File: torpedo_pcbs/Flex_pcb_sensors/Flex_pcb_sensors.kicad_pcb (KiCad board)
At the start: 2 copper layers, 38.2 x 23.8 mm, 9 parts, among them IC1 VL53L1CXV0FY_1, J1 Conn_01x04, J2 Conn_01x04, U1 MS583702BA01-50

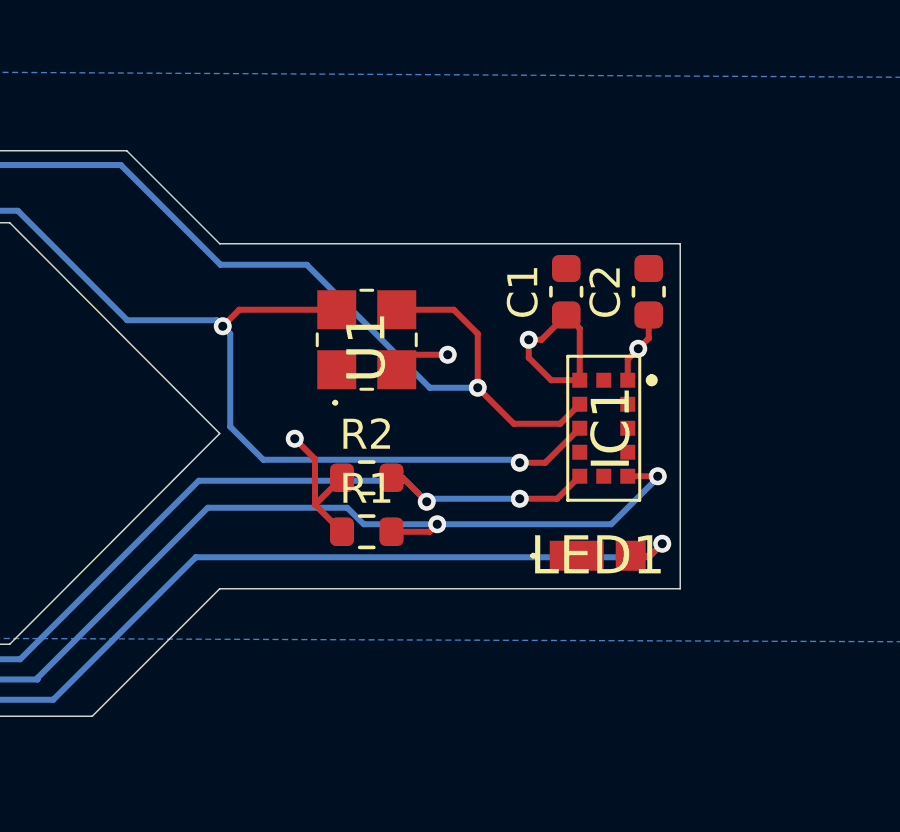
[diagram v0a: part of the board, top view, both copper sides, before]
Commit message: flex_pcb_updates
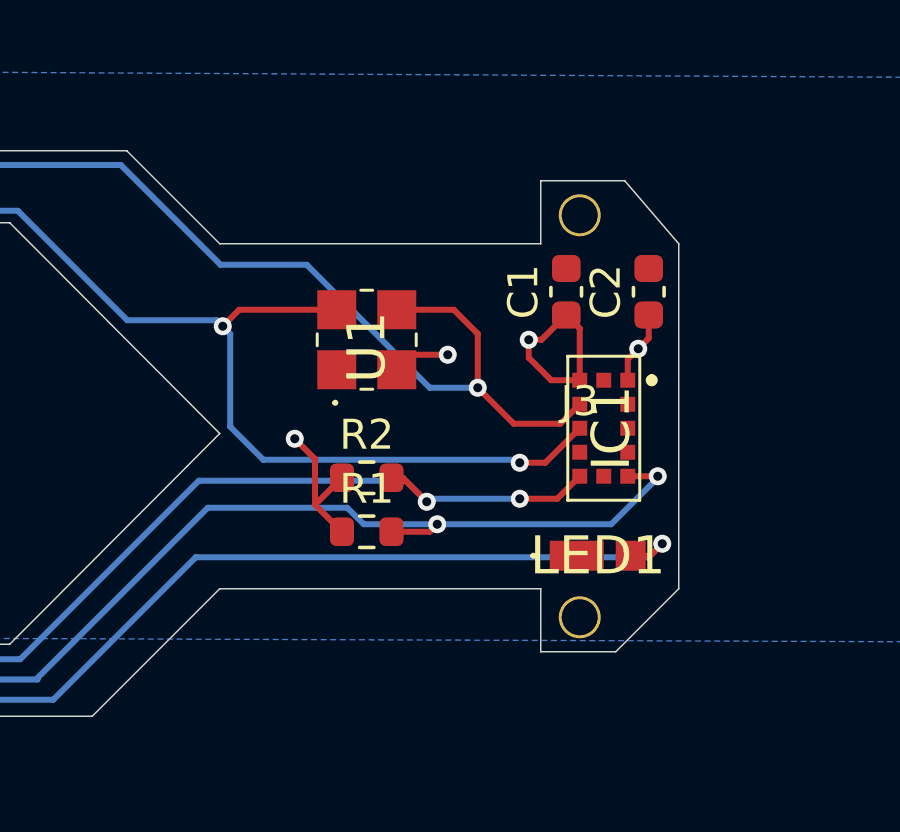
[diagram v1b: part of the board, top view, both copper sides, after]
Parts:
- added J3: mounting, MountingEquipment:small mounting holes, F.Cu at (171.8, 79.5)
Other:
- board size 38.2 x 23.8 mm -> 38.1 x 23.8 mm
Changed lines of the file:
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@@
 	(net 8 "unconnected-(J1-Pin_4-Pad4)")
 	(net 9 "Net-(J1-Pin_3)")
+	(footprint "MountingEquipment:small mounting holes"
+		(layer "F.Cu")
+		(at 171.8 79.45)
+		(property "Reference" "J3"
+			(at 0 -0.5 0)
+			(unlocked yes)
+			(layer "F.SilkS")
+			(effects
+				(font
+					(size 1 1)
+					(thickness 0.1)
+				)
+			)
+		)
+		(property "Value" "mounting"
+			(at 0 1 0)
+			(unlocked yes)
+			(layer "F.Fab")
+			(effects
+				(font
+					(size 1 1)
+					(thickness 0.15)
+				)
+			)
+		)
+		(property "Footprint" "MountingEquipment:small mounting holes"
+			(at 0 0 0)
+			(unlocked yes)
+			(layer "F.Fab")
+			(hide yes)
+			(effects
+				(font
+					(size 1 1)
+					(thickness 0.15)
+				)
+			)
+		)
+		(property "Datasheet" ""
+			(at 0 0 0)
+			(unlocked yes)
+			(layer "F.Fab")
+			(hide yes)
+			(effects
+				(font
+					(size 1 1)
+					(thickness 0.15)
+				)
+			)
+		)
+		(property "Description" "Generic connector, single row, 01x02, script generated (kicad-library-utils/schlib/autogen/connector/)"
+			(at 0 0 0)
+			(unlocked yes)
+			(layer "F.Fab")
+			(hide yes)
+			(effects
+				(font
+					(size 1 1)
+					(thickness 0.15)
+				)
+			)
+		)
+		(property ki_fp_filters "Connector*:*_1x??_*")
+		(sheetname "Root")
+		(sheetfile "Flex_pcb_sensors.kicad_sch")
+		(attr through_hole)
+		(fp_text user "${REFERENCE}"
+			(at 0 2.5 0)
+			(unlocked yes)
+			(layer "F.Fab")
+			(effects
+				(font
+					(size 1 1)
+					(thickness 0.15)
+				)
+			)
+		)
+		(pad "1" thru_hole circle
+			(at 0 -6.7)
+			(size 1.4 1.4)
+			(drill 1.2)
+			(layers "*.Cu" "*.Mask")
+			(remove_unused_layers no)
+			(net 4 "GND")
+			(pinfunction "Pin_1")
+			(pintype "passive")
+			(thermal_bridge_angle 90)
+		)
+		(pad "2" thru_hole circle
+			(at 0 6.7)
+			(size 1.4 1.4)
+			(drill 1.2)
+			(layers "*.Cu" "*.Mask")
+			(remove_unused_layers no)
+			(net 4 "GND")
+			(pinfunction "Pin_2")
+			(pintype "passive")
+			(thermal_bridge_angle 90)
+		)
+	)
 	(footprint "SamacSys_Parts:MS583702BA0150"
 		(layer "F.Cu")
@@
 		(tags "LED")
 		(property "Reference" "LED1"
-			(at 0 0 360)
+			(at 0 0 0)
 			(layer "F.SilkS")
 			(effects
@@
 		)
 		(property "Value" "158301260A"
-			(at 0 0 360)
+			(at 0 0 0)
 			(layer "F.SilkS")
 			(hide yes)
@@
 		)
 		(fp_line
-			(start -2.600001 1.7)
+			(start -2.6 -1.7)
+			(end 2.6 -1.7)
+			(stroke
+				(width 0.1)
+				(type solid)
+			)
+			(layer "F.CrtYd")
+		)
+		(fp_line
+			(start -2.6 1.7)
 			(end -2.6 -1.7)
 			(stroke
@@
 		)
 		(fp_line
-			(start -2.6 -1.7)
-			(end 2.600001 -1.7)
+			(start 2.6 -1.7)
+			(end 2.6 1.7)
 			(stroke
 				(width 0.1)
@@
 		(fp_line
 			(start 2.6 1.7)
-			(end -2.600001 1.7)
-			(stroke
-				(width 0.1)
-				(type solid)
-			)
-			(layer "F.CrtYd")
-		)
-		(fp_line
-			(start 2.600001 -1.7)
-			(end 2.6 1.7)
+			(end -2.6 1.7)
 			(stroke
 				(width 0.1)
@@
 		)
 		(fp_text user "${REFERENCE}"
-			(at 0 0 360)
+			(at 0 0 0)
 			(layer "F.Fab")
 			(effects
@@
 		)
 		(pad "2" smd rect
-			(at 1.099999 0.000002)
+			(at 1.1 0)
 			(size 1 1)
 			(layers "F.Cu" "F.Paste" "F.Mask")
@@
 			(pintype "passive")
 		)
-		(model "${KIPRJMOD}/SamacSys_Parts.3dshapes/158301260A.stp"
+		(model "\\\\Mac\\Home\\Ram\\Autonomous-Torpedo\\torpedo_pcbs\\Flex_pcb_sensors\\SamacSys_Parts.3dshapes\\158301260A.stp"
 			(offset
 				(xyz 0 0 0)
@@
 			(xy 148.35 70.6) (xy 145.875 68.125) (xy 137 68.125) (xy 137 70.525) (xy 144.125 70.525) (xy 146.55 73)
 			(xy 152.8 73) (xy 159.8 80.025) (xy 152.8 87.05) (xy 146.55 87.05) (xy 144.075 89.525) (xy 137 89.525)
-			(xy 137 91.925) (xy 145.825 91.925) (xy 148.3 89.45) (xy 155.55 89.45) (xy 159.8 85.2) (xy 175.15 85.2)
-			(xy 175.15 73.7) (xy 159.8 73.7) (xy 156.7 70.6)
+			(xy 137 91.925) (xy 145.825 91.925) (xy 148.3 89.45) (xy 155.55 89.45) (xy 159.8 85.2) (xy 170.5 85.2)
+			(xy 170.5 87.3) (xy 173 87.3) (xy 175.1 85.2) (xy 175.1 73.7) (xy 173.3 71.6) (xy 170.5 71.6) (xy 170.5 73.7)
+			(xy 159.8 73.7) (xy 156.7 70.6)
 		)
 		(stroke
@@
 		(layer "Edge.Cuts")
 	)
-	(gr_rect
-		(start 170.5 73.7)
-		(end 175.1 85.2)
+	(gr_poly
+		(pts
+			(xy 170.5 71.6) (xy 170.5 87.3) (xy 173 87.3) (xy 175.1 85.1) (xy 175.1 73.5) (xy 173.3 71.6)
+		)
 		(stroke
 			(width 0.1)
-			(type default)
+			(type solid)
 		)
 		(fill none)
@@
 	)
 	(gr_rect
-		(start 136.9 68.8)
-		(end 140.4 71.9)
+		(start 137 89.5)
+		(end 140.5 92)
+		(stroke
+			(width 0.1)
+			(type default)
+		)
+		(fill none)
+		(layer "User.2")
+	)
+	(gr_rect
+		(start 137 68.1)
+		(end 140.5 70.6)
 		(stroke
 			(width 0.1)
@@
 	)
 	(gr_text "Plastic\nstiffner"
-		(at 137 75 0)
+		(at 137 95.3 0)
 		(layer "User.2")
 		(effects
+			(font
+				(size 1 1)
+				(thickness 0.15)
+			)
+			(justify left bottom)
+		)
+	)
+	(gr_text "Plastic\nstiffner"
+		(at 137 73.9 0)
+		(layer "User.2")
+		(effects
